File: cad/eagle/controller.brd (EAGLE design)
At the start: 53 x 51 mm, 15 parts, among them X1 100MIL_2POS, X2 100MIL_2POS, X3 T821_10, X4 T821_10

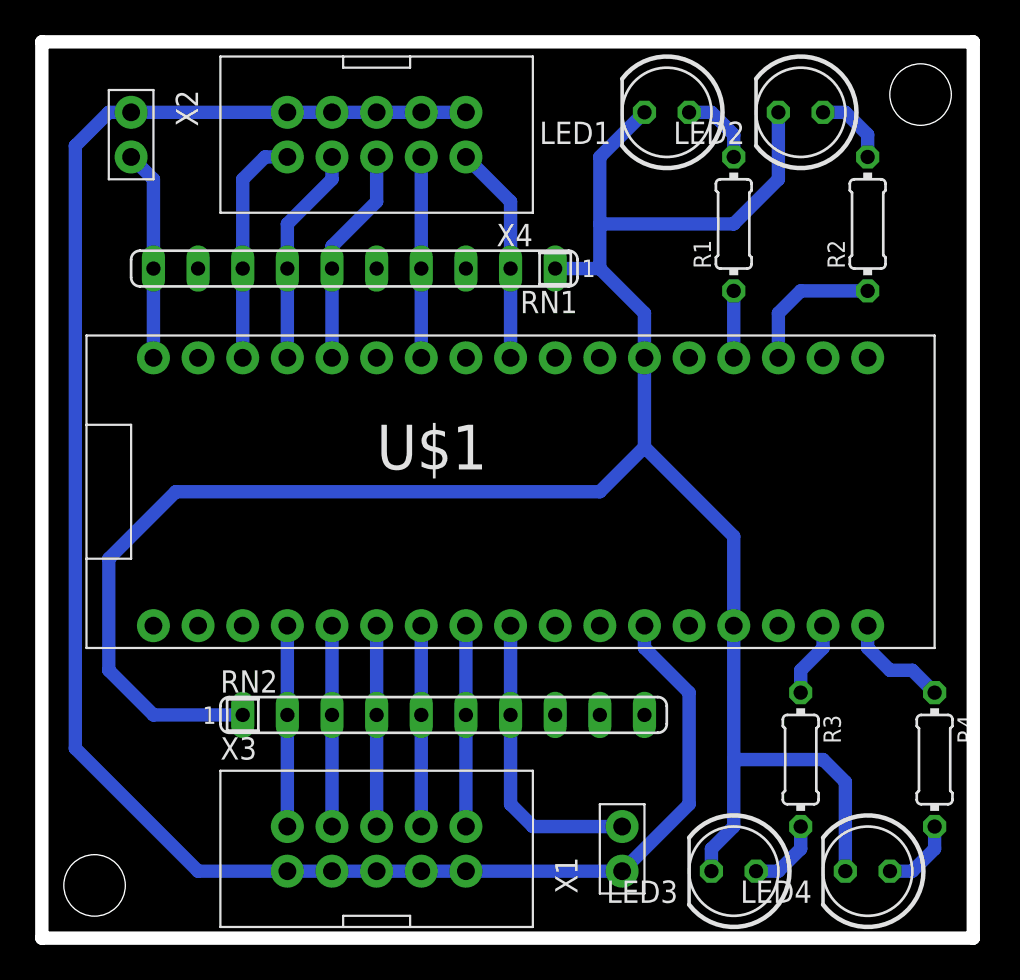
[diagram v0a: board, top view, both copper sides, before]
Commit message: new version *
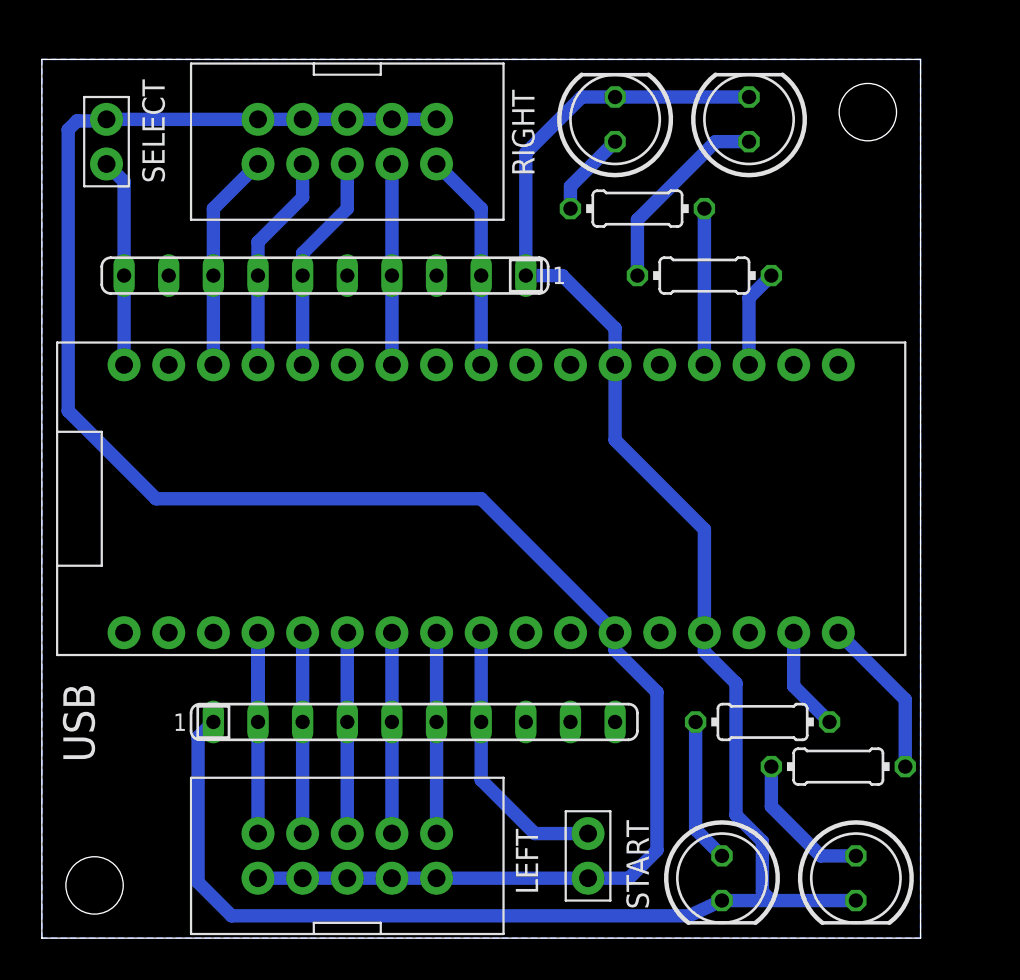
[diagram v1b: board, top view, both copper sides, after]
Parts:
- removed X1, X2: 100MIL_2POS, controller:100MIL_2POS
- removed X3, X4: T821_10, controller:T821_10
- added LEFT, RIGHT: T821_10, controller:T821_10
- added SELECT, START: 100MIL_2POS, controller:100MIL_2POS
- R1, R2, R3, R4: value 150 -> 100
- moved R2 9.74 mm to (37.7, 37.7), turned to 180 degrees
- moved R1 5.55 mm to (33.9, 41.5), turned to 180 degrees
- moved R4 5.49 mm to (45.3, 9.76), turned to 180 degrees
- moved R3 3.05 mm to (41.0, 12.3), turned to 180 degrees
- moved LED1 2.97 mm to (32.6, 46.6), turned to 90 degrees
- moved LED2 2.97 mm to (40.2, 46.6), turned to 90 degrees
- moved RN1 1.72 mm to (16.1, 37.7)
- moved U$1 1.72 mm to (25.0, 25.0)
- moved RN2 1.72 mm to (21.2, 12.3)
- moved LED4 0.78 mm to (46.3, 3.41), turned to 270 degrees
- moved LED3 0.78 mm to (38.7, 3.41), turned to 270 degrees
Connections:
- removed net N$10: RN1.9
- net +5V: now also LEFT.P$1, LEFT.P$3, LEFT.P$5, LEFT.P$7, LEFT.P$9, RIGHT.P$1, RIGHT.P$3, RIGHT.P$5, RIGHT.P$7, RIGHT.P$9, SELECT.P$1, START.P$1; no longer X1.P$1, X2.P$1, X3.P$1, X3.P$3, X3.P$5, X3.P$7, X3.P$9, X4.P$1, X4.P$3, X4.P$5, X4.P$7, X4.P$9
- net B0: now also LEFT.P$2; no longer X3.P$2
- net B1: now also LEFT.P$4; no longer X3.P$4
- net B10: now also RIGHT.P$10; no longer X4.P$10
- net B11: now also SELECT.P$2; no longer X2.P$2
- net B2: now also LEFT.P$6; no longer X3.P$6
- net B3: now also LEFT.P$8; no longer X3.P$8
- net B4: now also LEFT.P$10; no longer X3.P$10
- net B5: now also START.P$2; no longer X1.P$2
- net B6: now also RIGHT.P$2; no longer X4.P$2
- net B7: now also RIGHT.P$4; no longer X4.P$4
- net B8: now also RIGHT.P$6; no longer X4.P$6
- net B9: now also RIGHT.P$8; no longer X4.P$8
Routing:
- net GND: track 125.6 -> 111.5 mm
- net N$2: track 4.34 -> 11.4 mm
- net N$6: track 3.81 -> 8.89 mm
- net B0: track 11.4 -> 16.5 mm
- net N$4: track 4.34 -> 8.24 mm
- net N$3: track 4.34 -> 8.24 mm
- net N$8: track 6.13 -> 9.20 mm
- net N$7: track 8.15 -> 5.61 mm
- net +5V: track 107.9 -> 110.3 mm
- net N$9: track 4.34 -> 5.92 mm
- net B5: track 17.0 -> 15.7 mm
- net B10: track 13.2 -> 12.5 mm
- net N$1: track 4.34 -> 4.86 mm
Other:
- board size 53 x 51 mm -> 50 x 50 mm
- board text added: "USB"
